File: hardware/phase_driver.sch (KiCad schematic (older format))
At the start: 17 parts, among them Q1 BC817, Q2 BC817, Q3 BC817, Q4 BC807, Q5 BC817, Q6 BC807, Q7 AON7212, Q8 AON7212

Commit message: change to kicad 5
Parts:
- C1, C2: footprint Capacitors_SMD:C_0603 -> Capacitor_SMD:C_0603_1608Metric; symbol C -> Device:C
- Q1, Q2, Q3, Q5: footprint TO_SOT_Packages_SMD:SOT-23 -> Package_TO_SOT_SMD:SOT-23; symbol BC817 -> Transistor_BJT:BC817
- Q4, Q6: footprint TO_SOT_Packages_SMD:SOT-23 -> Package_TO_SOT_SMD:SOT-23; symbol BC807 -> Transistor_BJT:BC807
- Q7, Q8: symbol Q_NMOS_SGD -> Device:Q_NMOS_SGD
- R1, R2, R3, R4, R5, R6, R7: footprint Resistors_SMD:R_0603 -> Resistor_SMD:R_0603_1608Metric; symbol R -> Device:R

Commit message: smaller footprints
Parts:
- C1, C2: footprint Capacitor_SMD:C_0603_1608Metric -> _Generic:0603_Small
- Q1, Q2, Q3, Q4, Q5, Q6: footprint Package_TO_SOT_SMD:SOT-23 -> _Generic:SOT-23_Small
- Q7, Q8: footprint gmcontrol:DFN3x3A_8L_EP1_P -> _Generic:DFN3x3A_8L_EP1_P
- R1, R2, R3, R4, R5, R6, R7: footprint Resistor_SMD:R_0603_1608Metric -> _Generic:0603_Small
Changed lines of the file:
@@
 F 0 "Q5" H 7300 3825 50  0000 L CNN
 F 1 "BC817" H 7300 3750 50  0000 L CNN
-F 2 "Package_TO_SOT_SMD:SOT-23" H 7300 3675 50  0001 L CIN
+F 2 "_Generic:SOT-23_Small" H 7300 3675 50  0001 L CIN
 F 3 "" H 7100 3750 50  0001 L CNN
 	1    7100 3750
@@
 F 0 "Q2" H 6550 4425 50  0000 L CNN
 F 1 "BC817" H 6550 4350 50  0000 L CNN
-F 2 "Package_TO_SOT_SMD:SOT-23" H 6550 4275 50  0001 L CIN
+F 2 "_Generic:SOT-23_Small" H 6550 4275 50  0001 L CIN
 F 3 "" H 6350 4350 50  0001 L CNN
 	1    6350 4350
@@
 F 0 "Q6" H 7300 4425 50  0000 L CNN
 F 1 "BC807" H 7300 4350 50  0000 L CNN
-F 2 "Package_TO_SOT_SMD:SOT-23" H 7300 4275 50  0001 L CIN
+F 2 "_Generic:SOT-23_Small" H 7300 4275 50  0001 L CIN
 F 3 "" H 7100 4350 50  0001 L CNN
 	1    7100 4350
@@
 F 0 "R5" V 6530 3800 50  0000 C CNN
 F 1 "470" V 6450 3800 50  0000 C CNN
-F 2 "Resistor_SMD:R_0603_1608Metric" V 6380 3800 50  0001 C CNN
+F 2 "_Generic:0603_Small" V 6380 3800 50  0001 C CNN
 F 3 "" H 6450 3800 50  0001 C CNN
 	1    6450 3800
@@
 F 0 "R2" V 5880 4350 50  0000 C CNN
 F 1 "470" V 5800 4350 50  0000 C CNN
-F 2 "Resistor_SMD:R_0603_1608Metric" V 5730 4350 50  0001 C CNN
+F 2 "_Generic:0603_Small" V 5730 4350 50  0001 C CNN
 F 3 "" H 5800 4350 50  0001 C CNN
 	1    5800 4350
@@
 F 0 "Q8" H 7950 4100 50  0000 L CNN
 F 1 "AON7212" H 7950 4000 50  0000 L CNN
-F 2 "gmcontrol:DFN3x3A_8L_EP1_P" H 7950 4150 50  0001 C CNN
+F 2 "_Generic:DFN3x3A_8L_EP1_P" H 7950 4150 50  0001 C CNN
 F 3 "" H 7750 4050 50  0001 C CNN
 	1    7750 4050
@@
 F 0 "Q3" H 7300 1625 50  0000 L CNN
 F 1 "BC817" H 7300 1550 50  0000 L CNN
-F 2 "Package_TO_SOT_SMD:SOT-23" H 7300 1475 50  0001 L CIN
+F 2 "_Generic:SOT-23_Small" H 7300 1475 50  0001 L CIN
 F 3 "" H 7100 1550 50  0001 L CNN
 	1    7100 1550
@@
 F 0 "Q1" H 6550 2225 50  0000 L CNN
 F 1 "BC817" H 6550 2150 50  0000 L CNN
-F 2 "Package_TO_SOT_SMD:SOT-23" H 6550 2075 50  0001 L CIN
+F 2 "_Generic:SOT-23_Small" H 6550 2075 50  0001 L CIN
 F 3 "" H 6350 2150 50  0001 L CNN
 	1    6350 2150
@@
 F 0 "Q4" H 7300 2225 50  0000 L CNN
 F 1 "BC807" H 7300 2150 50  0000 L CNN
-F 2 "Package_TO_SOT_SMD:SOT-23" H 7300 2075 50  0001 L CIN
+F 2 "_Generic:SOT-23_Small" H 7300 2075 50  0001 L CIN
 F 3 "" H 7100 2150 50  0001 L CNN
 	1    7100 2150
@@
 F 0 "R3" V 6530 1600 50  0000 C CNN
 F 1 "470" V 6450 1600 50  0000 C CNN
-F 2 "Resistor_SMD:R_0603_1608Metric" V 6380 1600 50  0001 C CNN
+F 2 "_Generic:0603_Small" V 6380 1600 50  0001 C CNN
 F 3 "" H 6450 1600 50  0001 C CNN
 	1    6450 1600
@@
 F 0 "R1" V 5880 2150 50  0000 C CNN
 F 1 "470" V 5800 2150 50  0000 C CNN
-F 2 "Resistor_SMD:R_0603_1608Metric" V 5730 2150 50  0001 C CNN
+F 2 "_Generic:0603_Small" V 5730 2150 50  0001 C CNN
 F 3 "" H 5800 2150 50  0001 C CNN
 	1    5800 2150
@@
 F 0 "Q7" H 7950 1900 50  0000 L CNN
 F 1 "AON7212" H 7950 1800 50  0000 L CNN
-F 2 "gmcontrol:DFN3x3A_8L_EP1_P" H 7950 1950 50  0001 C CNN
+F 2 "_Generic:DFN3x3A_8L_EP1_P" H 7950 1950 50  0001 C CNN
 F 3 "" H 7750 1850 50  0001 C CNN
 	1    7750 1850
@@
 F 0 "R4" V 6530 2700 50  0000 C CNN
 F 1 "100" V 6450 2700 50  0000 C CNN
-F 2 "Resistor_SMD:R_0603_1608Metric" V 6380 2700 50  0001 C CNN
+F 2 "_Generic:0603_Small" V 6380 2700 50  0001 C CNN
 F 3 "" H 6450 2700 50  0001 C CNN
 	1    6450 2700
@@
 F 0 "R6" V 8830 3450 50  0000 C CNN
 F 1 "10k" V 8750 3450 50  0000 C CNN
-F 2 "Resistor_SMD:R_0603_1608Metric" V 8680 3450 50  0001 C CNN
+F 2 "_Generic:0603_Small" V 8680 3450 50  0001 C CNN
 F 3 "" H 8750 3450 50  0001 C CNN
 	1    8750 3450
@@
 F 0 "R7" V 8830 3950 50  0000 C CNN
 F 1 "1k" V 8750 3950 50  0000 C CNN
-F 2 "Resistor_SMD:R_0603_1608Metric" V 8680 3950 50  0001 C CNN
+F 2 "_Generic:0603_Small" V 8680 3950 50  0001 C CNN
 F 3 "" H 8750 3950 50  0001 C CNN
 	1    8750 3950
@@
 F 0 "C1" H 6075 3900 50  0000 L CNN
 F 1 "1u" H 6075 3700 50  0000 L CNN
-F 2 "Capacitor_SMD:C_0603_1608Metric" H 6088 3650 50  0001 C CNN
+F 2 "_Generic:0603_Small" H 6088 3650 50  0001 C CNN
 F 3 "" H 6050 3800 50  0001 C CNN
 	1    6050 3800
@@
 F 0 "C2" H 6125 1700 50  0000 L CNN
 F 1 "1u" H 6125 1500 50  0000 L CNN
-F 2 "Capacitor_SMD:C_0603_1608Metric" H 6138 1450 50  0001 C CNN
+F 2 "_Generic:0603_Small" H 6138 1450 50  0001 C CNN
 F 3 "" H 6100 1600 50  0001 C CNN
 	1    6100 1600

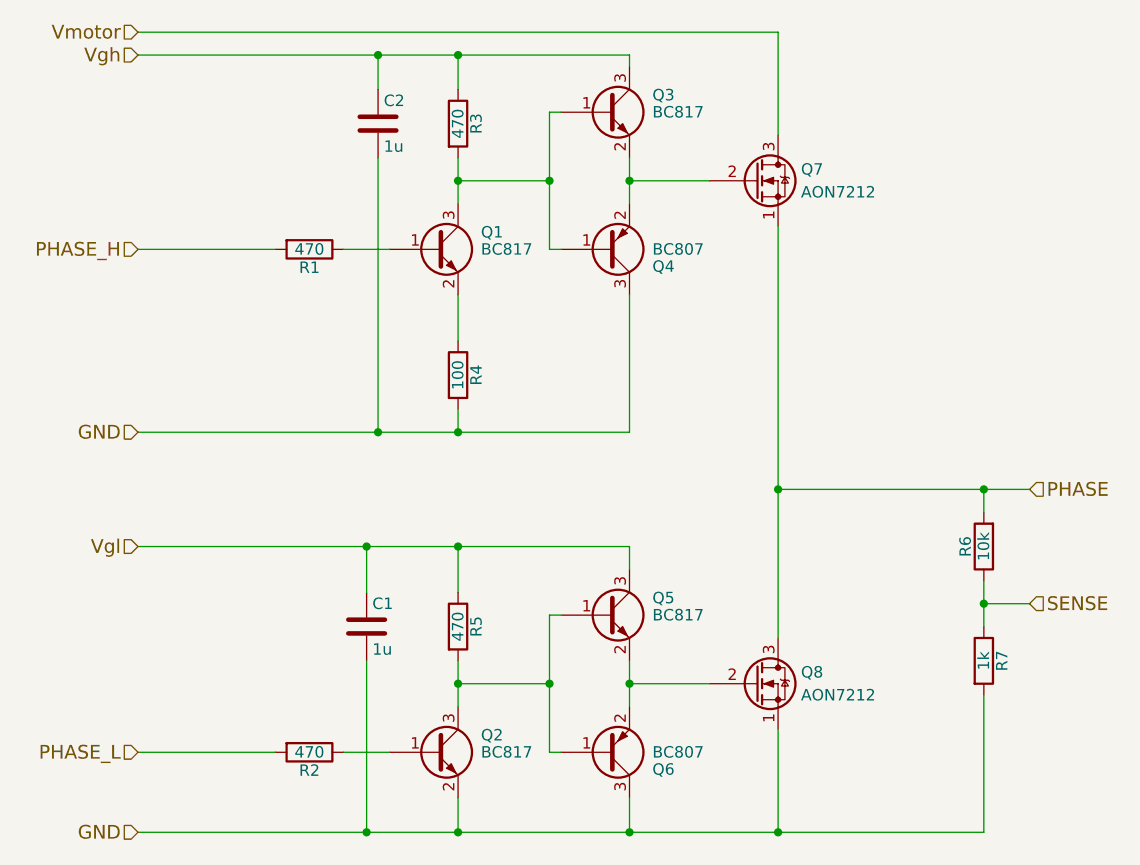
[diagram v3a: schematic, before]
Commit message: basic layout
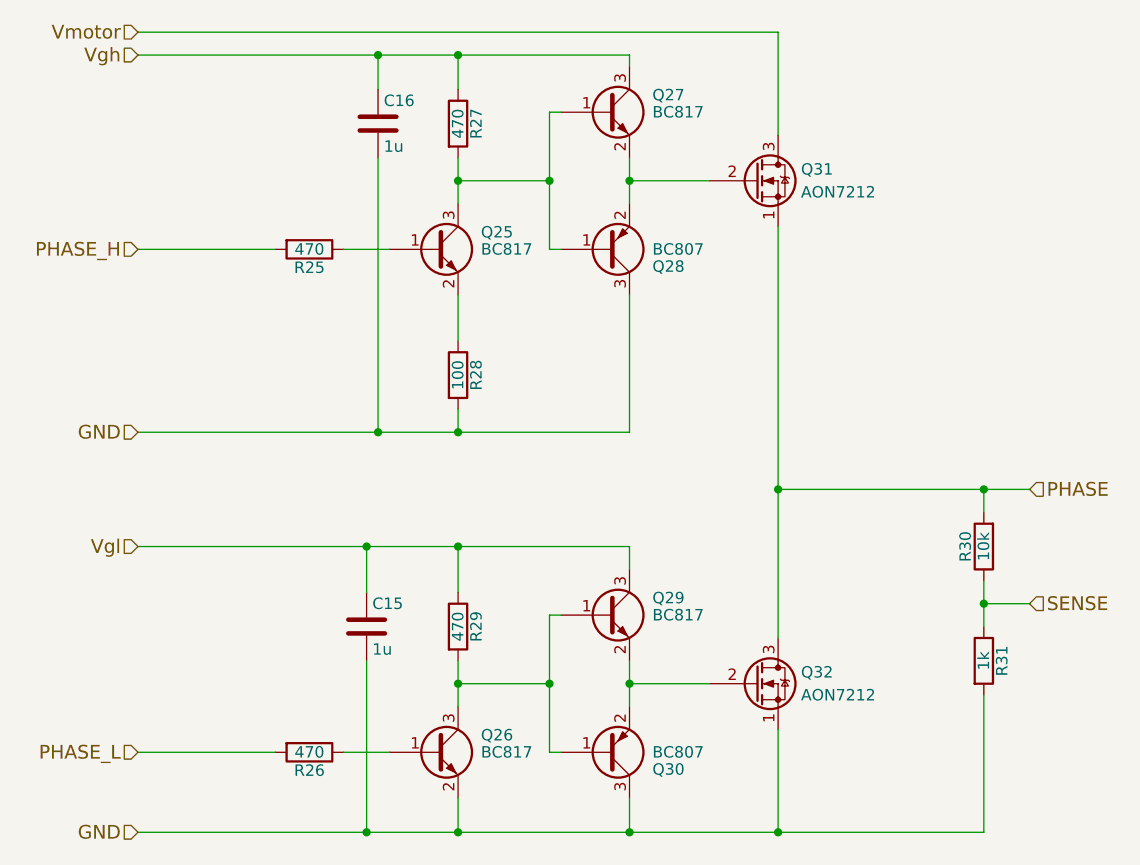
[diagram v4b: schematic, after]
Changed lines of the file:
@@
 AR Path="/5AEA2A43/5AE6CAAE" Ref="Q21"  Part="1"
 AR Path="/5AEA319E/5AE6CAAE" Ref="Q29"  Part="1"
-F 0 "Q5" H 7300 3825 50  0000 L CNN
+F 0 "Q29" H 7300 3825 50  0000 L CNN
 F 1 "BC817" H 7300 3750 50  0000 L CNN
 F 2 "_Generic:SOT-23_Small" H 7300 3675 50  0001 L CIN
@@
 AR Path="/5AEA2A43/5AE6CB43" Ref="Q18"  Part="1"
 AR Path="/5AEA319E/5AE6CB43" Ref="Q26"  Part="1"
-F 0 "Q2" H 6550 4425 50  0000 L CNN
+F 0 "Q26" H 6550 4425 50  0000 L CNN
 F 1 "BC817" H 6550 4350 50  0000 L CNN
 F 2 "_Generic:SOT-23_Small" H 6550 4275 50  0001 L CIN
@@
 AR Path="/5AEA2A43/5AE6CB8C" Ref="Q22"  Part="1"
 AR Path="/5AEA319E/5AE6CB8C" Ref="Q30"  Part="1"
-F 0 "Q6" H 7300 4425 50  0000 L CNN
+F 0 "Q30" H 7300 4425 50  0000 L CNN
 F 1 "BC807" H 7300 4350 50  0000 L CNN
 F 2 "_Generic:SOT-23_Small" H 7300 4275 50  0001 L CIN
@@
 AR Path="/5AEA2A43/5AE6CC83" Ref="R22"  Part="1"
 AR Path="/5AEA319E/5AE6CC83" Ref="R29"  Part="1"
-F 0 "R5" V 6530 3800 50  0000 C CNN
+F 0 "R29" V 6530 3800 50  0000 C CNN
 F 1 "470" V 6450 3800 50  0000 C CNN
 F 2 "_Generic:0603_Small" V 6380 3800 50  0001 C CNN
@@
 AR Path="/5AEA2A43/5AE6CCF2" Ref="R19"  Part="1"
 AR Path="/5AEA319E/5AE6CCF2" Ref="R26"  Part="1"
-F 0 "R2" V 5880 4350 50  0000 C CNN
+F 0 "R26" V 5880 4350 50  0000 C CNN
 F 1 "470" V 5800 4350 50  0000 C CNN
 F 2 "_Generic:0603_Small" V 5730 4350 50  0001 C CNN
@@
 AR Path="/5AEA2A43/5AE6CEBE" Ref="Q24"  Part="1"
 AR Path="/5AEA319E/5AE6CEBE" Ref="Q32"  Part="1"
-F 0 "Q8" H 7950 4100 50  0000 L CNN
+F 0 "Q32" H 7950 4100 50  0000 L CNN
 F 1 "AON7212" H 7950 4000 50  0000 L CNN
 F 2 "_Generic:DFN3x3A_8L_EP1_P" H 7950 4150 50  0001 C CNN
@@
 AR Path="/5AEA2A43/5AE6DEA8" Ref="Q19"  Part="1"
 AR Path="/5AEA319E/5AE6DEA8" Ref="Q27"  Part="1"
-F 0 "Q3" H 7300 1625 50  0000 L CNN
+F 0 "Q27" H 7300 1625 50  0000 L CNN
 F 1 "BC817" H 7300 1550 50  0000 L CNN
 F 2 "_Generic:SOT-23_Small" H 7300 1475 50  0001 L CIN
@@
 AR Path="/5AEA2A43/5AE6DEAF" Ref="Q17"  Part="1"
 AR Path="/5AEA319E/5AE6DEAF" Ref="Q25"  Part="1"
-F 0 "Q1" H 6550 2225 50  0000 L CNN
+F 0 "Q25" H 6550 2225 50  0000 L CNN
 F 1 "BC817" H 6550 2150 50  0000 L CNN
 F 2 "_Generic:SOT-23_Small" H 6550 2075 50  0001 L CIN
@@
 AR Path="/5AEA2A43/5AE6DEB6" Ref="Q20"  Part="1"
 AR Path="/5AEA319E/5AE6DEB6" Ref="Q28"  Part="1"
-F 0 "Q4" H 7300 2225 50  0000 L CNN
+F 0 "Q28" H 7300 2225 50  0000 L CNN
 F 1 "BC807" H 7300 2150 50  0000 L CNN
 F 2 "_Generic:SOT-23_Small" H 7300 2075 50  0001 L CIN
@@
 AR Path="/5AEA2A43/5AE6DEBD" Ref="R20"  Part="1"
 AR Path="/5AEA319E/5AE6DEBD" Ref="R27"  Part="1"
-F 0 "R3" V 6530 1600 50  0000 C CNN
+F 0 "R27" V 6530 1600 50  0000 C CNN
 F 1 "470" V 6450 1600 50  0000 C CNN
 F 2 "_Generic:0603_Small" V 6380 1600 50  0001 C CNN
@@
 AR Path="/5AEA2A43/5AE6DEC4" Ref="R18"  Part="1"
 AR Path="/5AEA319E/5AE6DEC4" Ref="R25"  Part="1"
-F 0 "R1" V 5880 2150 50  0000 C CNN
+F 0 "R25" V 5880 2150 50  0000 C CNN
 F 1 "470" V 5800 2150 50  0000 C CNN
 F 2 "_Generic:0603_Small" V 5730 2150 50  0001 C CNN
@@
 AR Path="/5AEA2A43/5AE6DEDD" Ref="Q23"  Part="1"
 AR Path="/5AEA319E/5AE6DEDD" Ref="Q31"  Part="1"
-F 0 "Q7" H 7950 1900 50  0000 L CNN
+F 0 "Q31" H 7950 1900 50  0000 L CNN
 F 1 "AON7212" H 7950 1800 50  0000 L CNN
 F 2 "_Generic:DFN3x3A_8L_EP1_P" H 7950 1950 50  0001 C CNN
@@
 AR Path="/5AEA2A43/5AE6E0AE" Ref="R21"  Part="1"
 AR Path="/5AEA319E/5AE6E0AE" Ref="R28"  Part="1"
-F 0 "R4" V 6530 2700 50  0000 C CNN
+F 0 "R28" V 6530 2700 50  0000 C CNN
 F 1 "100" V 6450 2700 50  0000 C CNN
 F 2 "_Generic:0603_Small" V 6380 2700 50  0001 C CNN
@@
 AR Path="/5AEA2A43/5AE87A58" Ref="R23"  Part="1"
 AR Path="/5AEA319E/5AE87A58" Ref="R30"  Part="1"
-F 0 "R6" V 8830 3450 50  0000 C CNN
+F 0 "R30" V 8830 3450 50  0000 C CNN
 F 1 "10k" V 8750 3450 50  0000 C CNN
 F 2 "_Generic:0603_Small" V 8680 3450 50  0001 C CNN
@@
 AR Path="/5AEA2A43/5AE87B6A" Ref="R24"  Part="1"
 AR Path="/5AEA319E/5AE87B6A" Ref="R31"  Part="1"
-F 0 "R7" V 8830 3950 50  0000 C CNN
+F 0 "R31" V 8830 3950 50  0000 C CNN
 F 1 "1k" V 8750 3950 50  0000 C CNN
 F 2 "_Generic:0603_Small" V 8680 3950 50  0001 C CNN
@@
 AR Path="/5AEA2A43/5AE9E83C" Ref="C13"  Part="1"
 AR Path="/5AEA319E/5AE9E83C" Ref="C15"  Part="1"
-F 0 "C1" H 6075 3900 50  0000 L CNN
+F 0 "C15" H 6075 3900 50  0000 L CNN
 F 1 "1u" H 6075 3700 50  0000 L CNN
 F 2 "_Generic:0603_Small" H 6088 3650 50  0001 C CNN
@@
 AR Path="/5AEA2A43/5AE9EAA8" Ref="C14"  Part="1"
 AR Path="/5AEA319E/5AE9EAA8" Ref="C16"  Part="1"
-F 0 "C2" H 6125 1700 50  0000 L CNN
+F 0 "C16" H 6125 1700 50  0000 L CNN
 F 1 "1u" H 6125 1500 50  0000 L CNN
 F 2 "_Generic:0603_Small" H 6138 1450 50  0001 C CNN

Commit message: stm layout
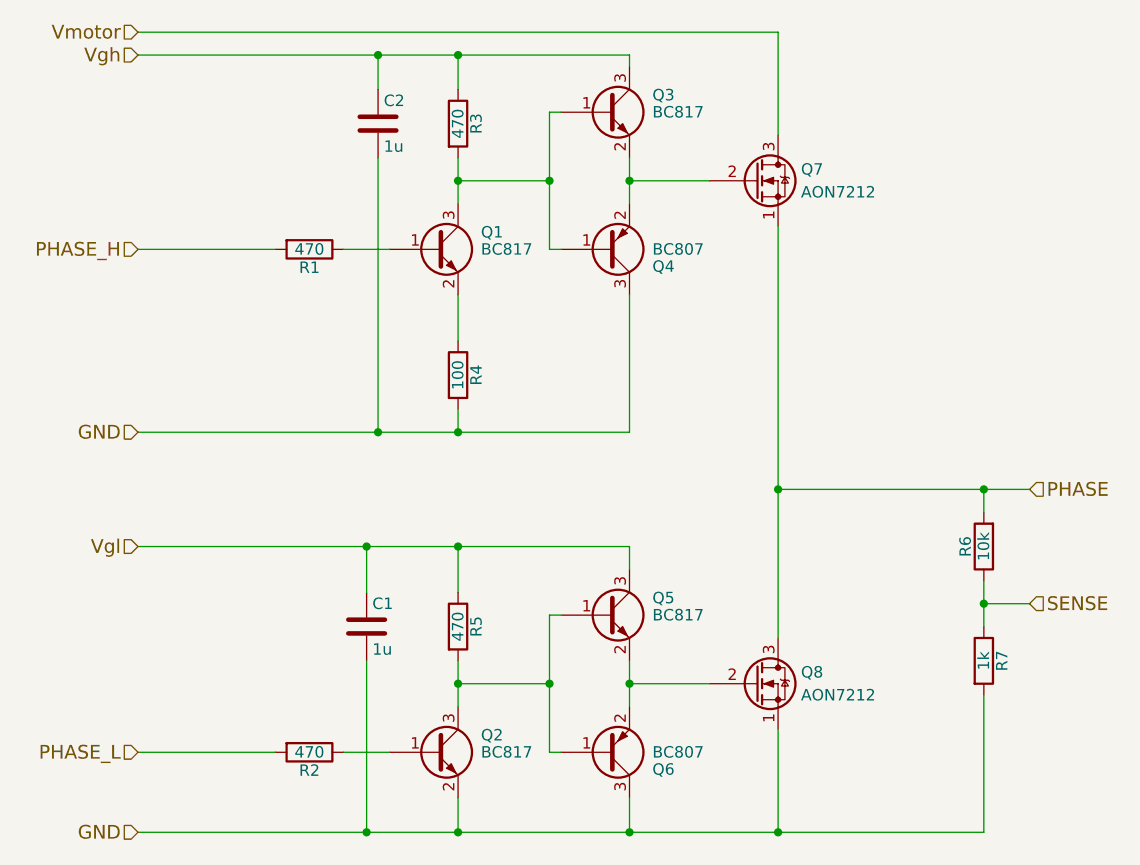
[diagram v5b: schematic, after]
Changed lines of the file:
@@
 AR Path="/5AEA2A43/5AE6CAAE" Ref="Q21"  Part="1"
 AR Path="/5AEA319E/5AE6CAAE" Ref="Q29"  Part="1"
-F 0 "Q29" H 7300 3825 50  0000 L CNN
+F 0 "Q5" H 7300 3825 50  0000 L CNN
 F 1 "BC817" H 7300 3750 50  0000 L CNN
 F 2 "_Generic:SOT-23_Small" H 7300 3675 50  0001 L CIN
@@
 AR Path="/5AEA2A43/5AE6CB43" Ref="Q18"  Part="1"
 AR Path="/5AEA319E/5AE6CB43" Ref="Q26"  Part="1"
-F 0 "Q26" H 6550 4425 50  0000 L CNN
+F 0 "Q2" H 6550 4425 50  0000 L CNN
 F 1 "BC817" H 6550 4350 50  0000 L CNN
 F 2 "_Generic:SOT-23_Small" H 6550 4275 50  0001 L CIN
@@
 AR Path="/5AEA2A43/5AE6CB8C" Ref="Q22"  Part="1"
 AR Path="/5AEA319E/5AE6CB8C" Ref="Q30"  Part="1"
-F 0 "Q30" H 7300 4425 50  0000 L CNN
+F 0 "Q6" H 7300 4425 50  0000 L CNN
 F 1 "BC807" H 7300 4350 50  0000 L CNN
 F 2 "_Generic:SOT-23_Small" H 7300 4275 50  0001 L CIN
@@
 AR Path="/5AEA2A43/5AE6CC83" Ref="R22"  Part="1"
 AR Path="/5AEA319E/5AE6CC83" Ref="R29"  Part="1"
-F 0 "R29" V 6530 3800 50  0000 C CNN
+F 0 "R5" V 6530 3800 50  0000 C CNN
 F 1 "470" V 6450 3800 50  0000 C CNN
 F 2 "_Generic:0603_Small" V 6380 3800 50  0001 C CNN
@@
 AR Path="/5AEA2A43/5AE6CCF2" Ref="R19"  Part="1"
 AR Path="/5AEA319E/5AE6CCF2" Ref="R26"  Part="1"
-F 0 "R26" V 5880 4350 50  0000 C CNN
+F 0 "R2" V 5880 4350 50  0000 C CNN
 F 1 "470" V 5800 4350 50  0000 C CNN
 F 2 "_Generic:0603_Small" V 5730 4350 50  0001 C CNN
@@
 AR Path="/5AEA2A43/5AE6CEBE" Ref="Q24"  Part="1"
 AR Path="/5AEA319E/5AE6CEBE" Ref="Q32"  Part="1"
-F 0 "Q32" H 7950 4100 50  0000 L CNN
+F 0 "Q8" H 7950 4100 50  0000 L CNN
 F 1 "AON7212" H 7950 4000 50  0000 L CNN
 F 2 "_Generic:DFN3x3A_8L_EP1_P" H 7950 4150 50  0001 C CNN
@@
 AR Path="/5AEA2A43/5AE6DEA8" Ref="Q19"  Part="1"
 AR Path="/5AEA319E/5AE6DEA8" Ref="Q27"  Part="1"
-F 0 "Q27" H 7300 1625 50  0000 L CNN
+F 0 "Q3" H 7300 1625 50  0000 L CNN
 F 1 "BC817" H 7300 1550 50  0000 L CNN
 F 2 "_Generic:SOT-23_Small" H 7300 1475 50  0001 L CIN
@@
 AR Path="/5AEA2A43/5AE6DEAF" Ref="Q17"  Part="1"
 AR Path="/5AEA319E/5AE6DEAF" Ref="Q25"  Part="1"
-F 0 "Q25" H 6550 2225 50  0000 L CNN
+F 0 "Q1" H 6550 2225 50  0000 L CNN
 F 1 "BC817" H 6550 2150 50  0000 L CNN
 F 2 "_Generic:SOT-23_Small" H 6550 2075 50  0001 L CIN
@@
 AR Path="/5AEA2A43/5AE6DEB6" Ref="Q20"  Part="1"
 AR Path="/5AEA319E/5AE6DEB6" Ref="Q28"  Part="1"
-F 0 "Q28" H 7300 2225 50  0000 L CNN
+F 0 "Q4" H 7300 2225 50  0000 L CNN
 F 1 "BC807" H 7300 2150 50  0000 L CNN
 F 2 "_Generic:SOT-23_Small" H 7300 2075 50  0001 L CIN
@@
 AR Path="/5AEA2A43/5AE6DEBD" Ref="R20"  Part="1"
 AR Path="/5AEA319E/5AE6DEBD" Ref="R27"  Part="1"
-F 0 "R27" V 6530 1600 50  0000 C CNN
+F 0 "R3" V 6530 1600 50  0000 C CNN
 F 1 "470" V 6450 1600 50  0000 C CNN
 F 2 "_Generic:0603_Small" V 6380 1600 50  0001 C CNN
@@
 AR Path="/5AEA2A43/5AE6DEC4" Ref="R18"  Part="1"
 AR Path="/5AEA319E/5AE6DEC4" Ref="R25"  Part="1"
-F 0 "R25" V 5880 2150 50  0000 C CNN
+F 0 "R1" V 5880 2150 50  0000 C CNN
 F 1 "470" V 5800 2150 50  0000 C CNN
 F 2 "_Generic:0603_Small" V 5730 2150 50  0001 C CNN
@@
 AR Path="/5AEA2A43/5AE6DEDD" Ref="Q23"  Part="1"
 AR Path="/5AEA319E/5AE6DEDD" Ref="Q31"  Part="1"
-F 0 "Q31" H 7950 1900 50  0000 L CNN
+F 0 "Q7" H 7950 1900 50  0000 L CNN
 F 1 "AON7212" H 7950 1800 50  0000 L CNN
 F 2 "_Generic:DFN3x3A_8L_EP1_P" H 7950 1950 50  0001 C CNN
@@
 AR Path="/5AEA2A43/5AE6E0AE" Ref="R21"  Part="1"
 AR Path="/5AEA319E/5AE6E0AE" Ref="R28"  Part="1"
-F 0 "R28" V 6530 2700 50  0000 C CNN
+F 0 "R4" V 6530 2700 50  0000 C CNN
 F 1 "100" V 6450 2700 50  0000 C CNN
 F 2 "_Generic:0603_Small" V 6380 2700 50  0001 C CNN
@@
 AR Path="/5AEA2A43/5AE87A58" Ref="R23"  Part="1"
 AR Path="/5AEA319E/5AE87A58" Ref="R30"  Part="1"
-F 0 "R30" V 8830 3450 50  0000 C CNN
+F 0 "R6" V 8830 3450 50  0000 C CNN
 F 1 "10k" V 8750 3450 50  0000 C CNN
 F 2 "_Generic:0603_Small" V 8680 3450 50  0001 C CNN
@@
 AR Path="/5AEA2A43/5AE87B6A" Ref="R24"  Part="1"
 AR Path="/5AEA319E/5AE87B6A" Ref="R31"  Part="1"
-F 0 "R31" V 8830 3950 50  0000 C CNN
+F 0 "R7" V 8830 3950 50  0000 C CNN
 F 1 "1k" V 8750 3950 50  0000 C CNN
 F 2 "_Generic:0603_Small" V 8680 3950 50  0001 C CNN
@@
 AR Path="/5AEA2A43/5AE9E83C" Ref="C13"  Part="1"
 AR Path="/5AEA319E/5AE9E83C" Ref="C15"  Part="1"
-F 0 "C15" H 6075 3900 50  0000 L CNN
+F 0 "C1" H 6075 3900 50  0000 L CNN
 F 1 "1u" H 6075 3700 50  0000 L CNN
 F 2 "_Generic:0603_Small" H 6088 3650 50  0001 C CNN
@@
 AR Path="/5AEA2A43/5AE9EAA8" Ref="C14"  Part="1"
 AR Path="/5AEA319E/5AE9EAA8" Ref="C16"  Part="1"
-F 0 "C16" H 6125 1700 50  0000 L CNN
+F 0 "C2" H 6125 1700 50  0000 L CNN
 F 1 "1u" H 6125 1500 50  0000 L CNN
 F 2 "_Generic:0603_Small" H 6138 1450 50  0001 C CNN
